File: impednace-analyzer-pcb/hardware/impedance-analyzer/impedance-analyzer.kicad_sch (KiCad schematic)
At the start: 9 parts, among them J1 AD9833, J2 ADS1256_SPI, J3 ADS1256_AIN, J4 UNO_POWER, J5 UNO_ANALOG, J6 UNO_DIGITAL_LOW, J7 UNO_DIGITAL_HIGH, J8 PIEZO

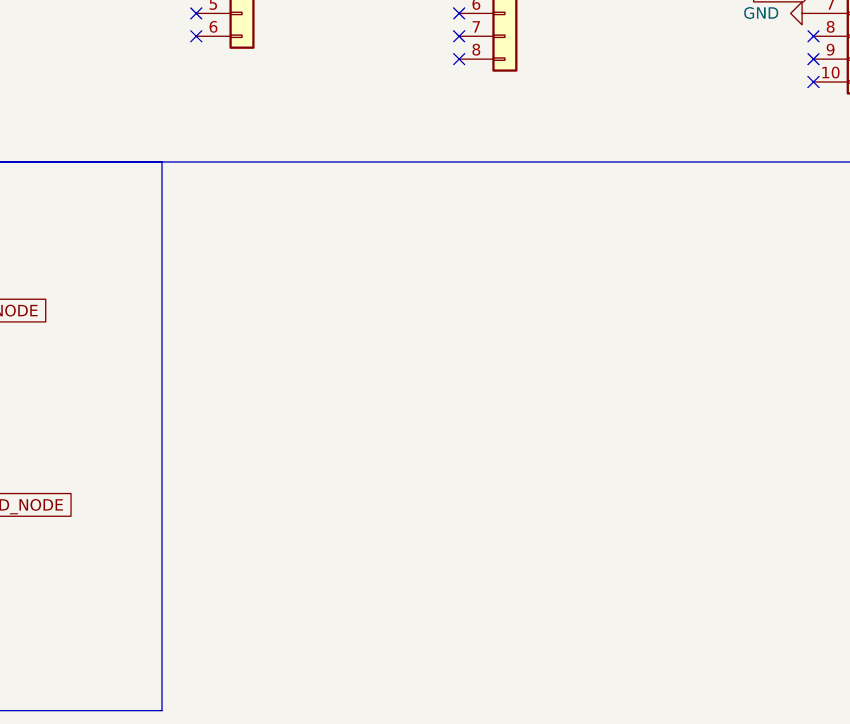
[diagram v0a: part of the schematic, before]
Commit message: pcb stuff
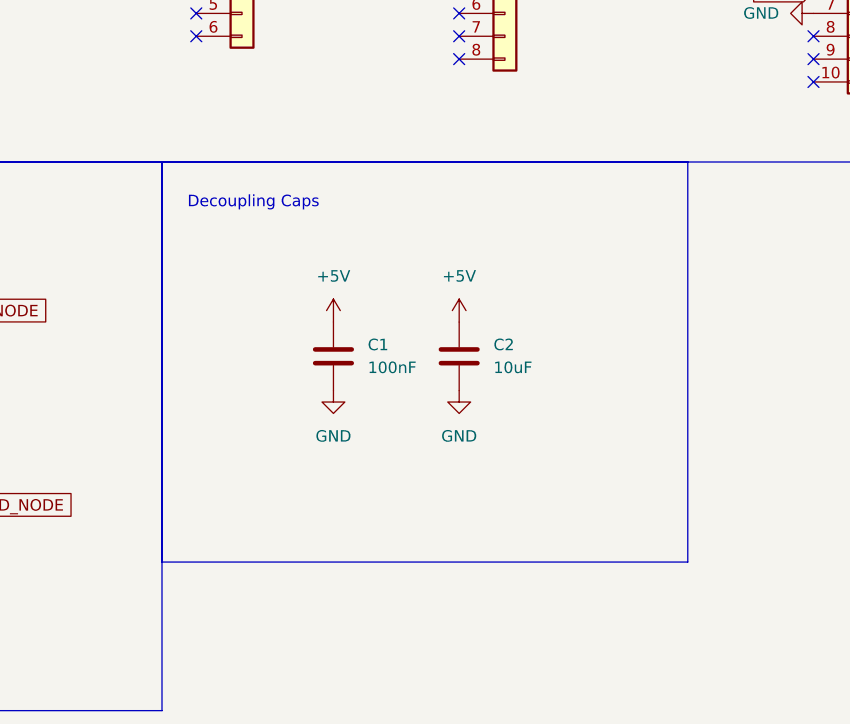
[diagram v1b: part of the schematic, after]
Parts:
- added C1: 100nF, Capacitor_SMD:C_0805_2012Metric_Pad1.18x1.45mm_HandSolder, symbol Device:C
- added C2: 10uF, Capacitor_SMD:C_0805_2012Metric_Pad1.18x1.45mm_HandSolder, symbol Device:C
- J1: footprint (none) -> Connector_PinSocket_2.54mm:PinSocket_1x07_P2.54mm_Vertical
- J2: footprint (none) -> Connector_PinSocket_2.54mm:PinSocket_1x08_P2.54mm_Vertical
- J3: footprint (none) -> Connector_PinSocket_2.54mm:PinSocket_2x08_P2.54mm_Vertical
- J4, J6: footprint (none) -> Connector_PinHeader_2.54mm:PinHeader_1x08_P2.54mm_Vertical
- J5: footprint (none) -> Connector_PinHeader_2.54mm:PinHeader_1x06_P2.54mm_Vertical
- J7: footprint (none) -> Connector_PinHeader_2.54mm:PinHeader_1x10_P2.54mm_Vertical
- J8: footprint (none) -> TerminalBlock:TerminalBlock_MaiXu_MX126-5.0-02P_1x02_P5.00mm
- RV1: footprint (none) -> Potentiometer_THT:Potentiometer_Bourns_3296W_Vertical
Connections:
- net +5V: now also C1.1, C2.1
- net GND: now also C1.2, C2.2
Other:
- note added: "Decoupling Caps"
